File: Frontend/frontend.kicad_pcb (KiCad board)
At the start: 4 copper layers, 100 x 100.2 mm, 364 parts, among them J1 VOCM, J10 SWD, J11 APWR, J2 BNC, J3 UMC, J4 UMC, J5 VOCM, J6 BNC, J7 UMC, J8 UMC, J9 PCIEx4 EDGE, K1 HE3600, K2 EE2-5NU, K3 HE3600, K4 HE3600, K5 EE2-5NU, K6 HE3600, Q1 ULN2003AD, U1 MCP9700T-E/TT, U10 ADA4817-1ACPZ, U11 MAX4567EEE, U12 MAX4567EEE, U13 MAX4567EEE, U14 AD8003ACPZ, U15 LMH6552SD, U16 MC33078DGK, U17 MAX5725AAUP, U18 STM32F030C8T, U19 MC33078DGK, U2 ADA4817-1ACPZ, U20 MC33078DGK, U21 MC33078DGK, U22 MC33078DGK, U23 LM317S, U24 MCP9700T-E/TT, U25 L78M05CDT, U26 TLV70233DSE, U27 MCP9700T-E/TT, U28 MC79M05CDT, U3 MAX4567EEE, U4 MAX4567EEE, U5 MAX4567EEE, U6 AD8003ACPZ, U7 LMH6552SD, U8 MC33078DGK, U9 MCP9700T-E/TT

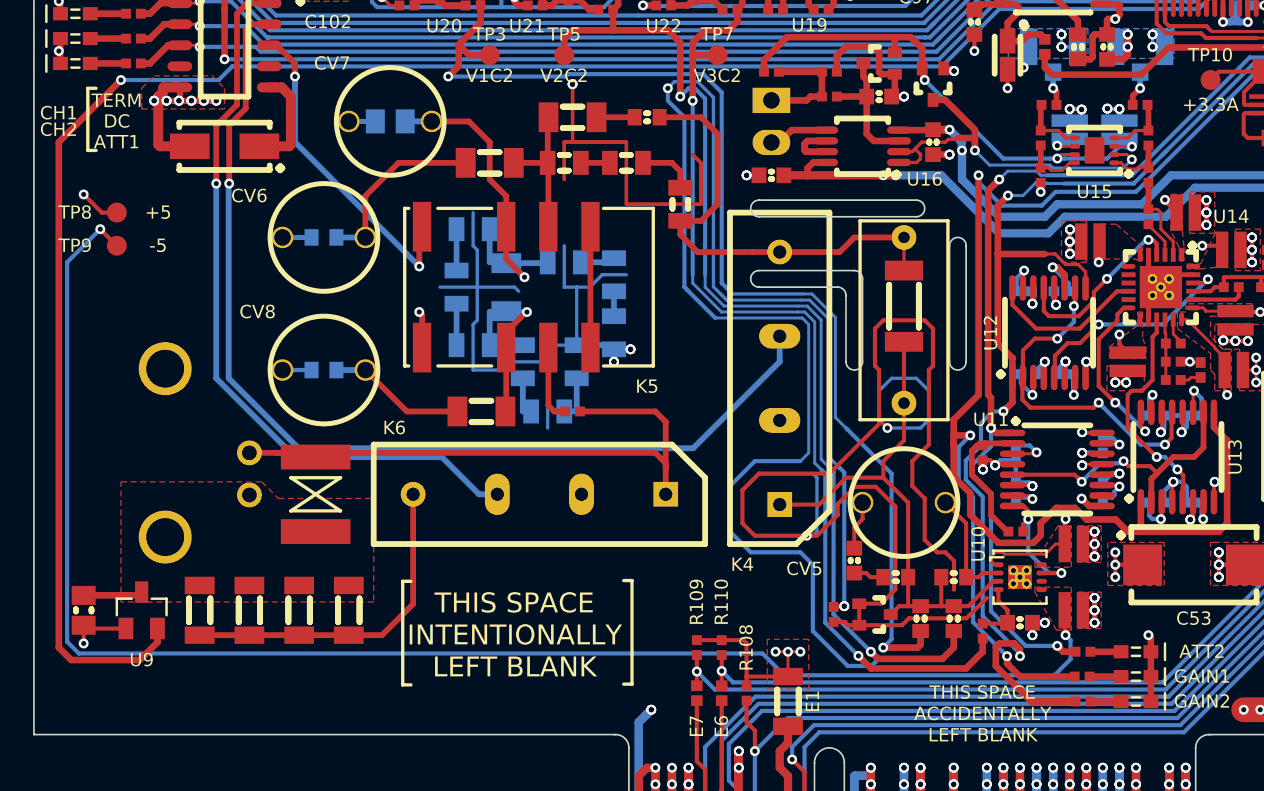
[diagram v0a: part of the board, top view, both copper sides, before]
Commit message: Schematic cleanup
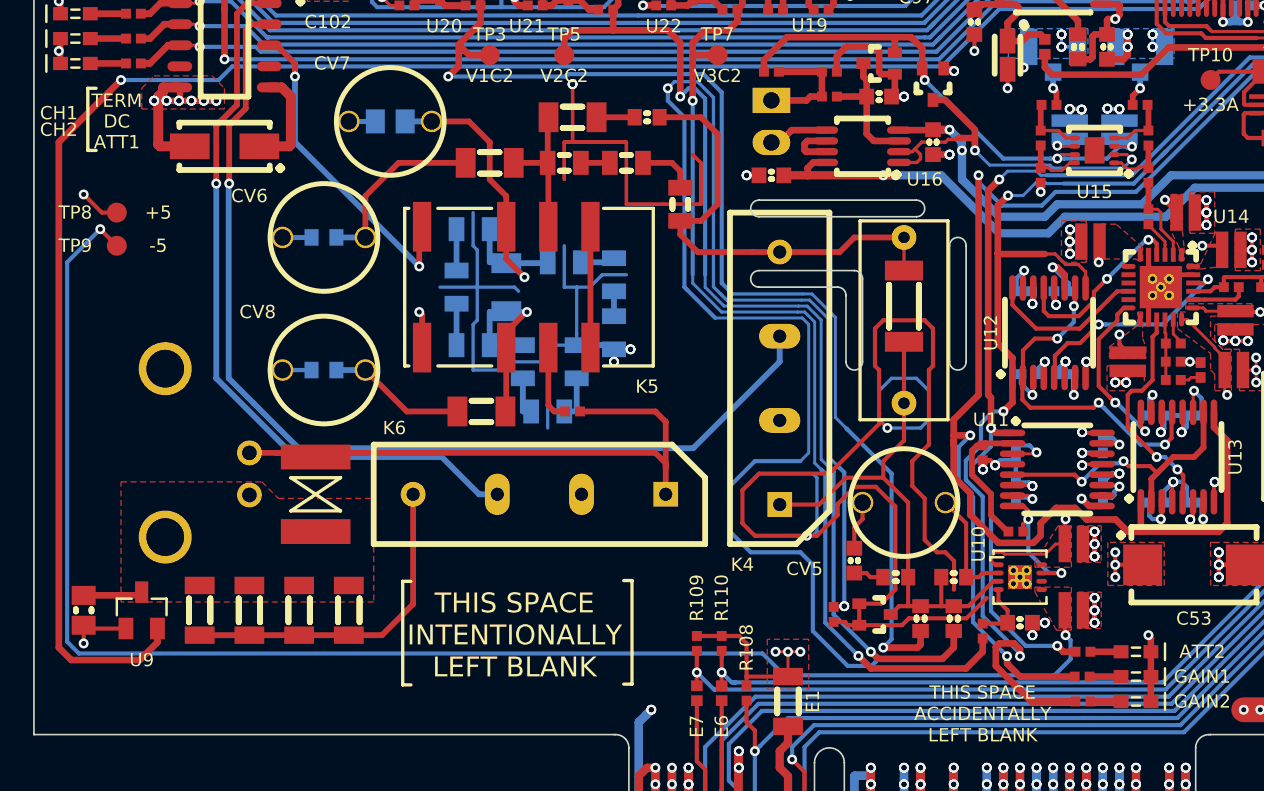
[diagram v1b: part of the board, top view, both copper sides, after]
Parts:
- U18: value STM32F030C8T -> STM32V030C8T
- moved R109 0.25 mm to (102.0, 103.5)
- moved R110 0.25 mm to (103.5, 103.5)
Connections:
- net /Microcontroller/#CSEXT renamed /Microcontroller/F_#SS
- net /Microcontroller/+5VMON renamed Net-(R90-Pad2)
- net /Microcontroller/-5VMON renamed Net-(R91-Pad2)
- net /Microcontroller/3V3ADC renamed Net-(C88-Pad1)
- net /Microcontroller/MISOEXT renamed /Microcontroller/F_MISO
- net /Microcontroller/MOSIEXT renamed /Microcontroller/F_MOSI
- net /Microcontroller/SCKEXT renamed /Microcontroller/F_SCK
- net /Microcontroller/TX renamed Net-(TP1-Pad1)
- E6 pad 1: Net-(E6-Pad1) -> /Microcontroller/SCL
- E6 pad 2: /Microcontroller/SCL -> /Microcontroller/F_SCL
- E7 pad 1: Net-(E7-Pad1) -> /Microcontroller/SDA
- E7 pad 2: /Microcontroller/SDA -> /Microcontroller/F_SDA
- J9 pad B5: Net-(E7-Pad1) -> /Microcontroller/SDA
- J9 pad B6: Net-(E6-Pad1) -> /Microcontroller/SCL
- R109 pad 2: /Microcontroller/SDA -> /Microcontroller/F_SDA
- R110 pad 2: /Microcontroller/SCL -> /Microcontroller/F_SCL
- U18 pad 21: /Microcontroller/SCL -> /Microcontroller/F_SCL
- U18 pad 22: /Microcontroller/SDA -> /Microcontroller/F_SDA
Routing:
- net /Microcontroller/F_SDA: track 0.00 -> 98.6 mm, vias 0 -> 2
- net /Microcontroller/F_SCL: track 0.00 -> 94.6 mm, vias 0 -> 2
- net /Microcontroller/SDA: track 98.4 -> 7.86 mm, vias 2 -> 0
- net /Microcontroller/SCL: track 94.2 -> 7.65 mm, vias 2 -> 0
- net Net-(E7-Pad1): track 7.86 -> 0.00 mm
- net Net-(E6-Pad1): track 7.65 -> 0.00 mm
